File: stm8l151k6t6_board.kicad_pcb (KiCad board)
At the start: 2 copper layers, 68.4 x 39.4 mm, 31 parts, among them J1 Conn_01x08, J2 Conn_01x08, J3 Conn_01x08, J4 Conn_01x08, J5 Conn_01x04, U1 USB_B_Micro, U2 TPMIC5504, U3 STM8L151K6T6, Y1 8MHz, Y2 32K768Hz

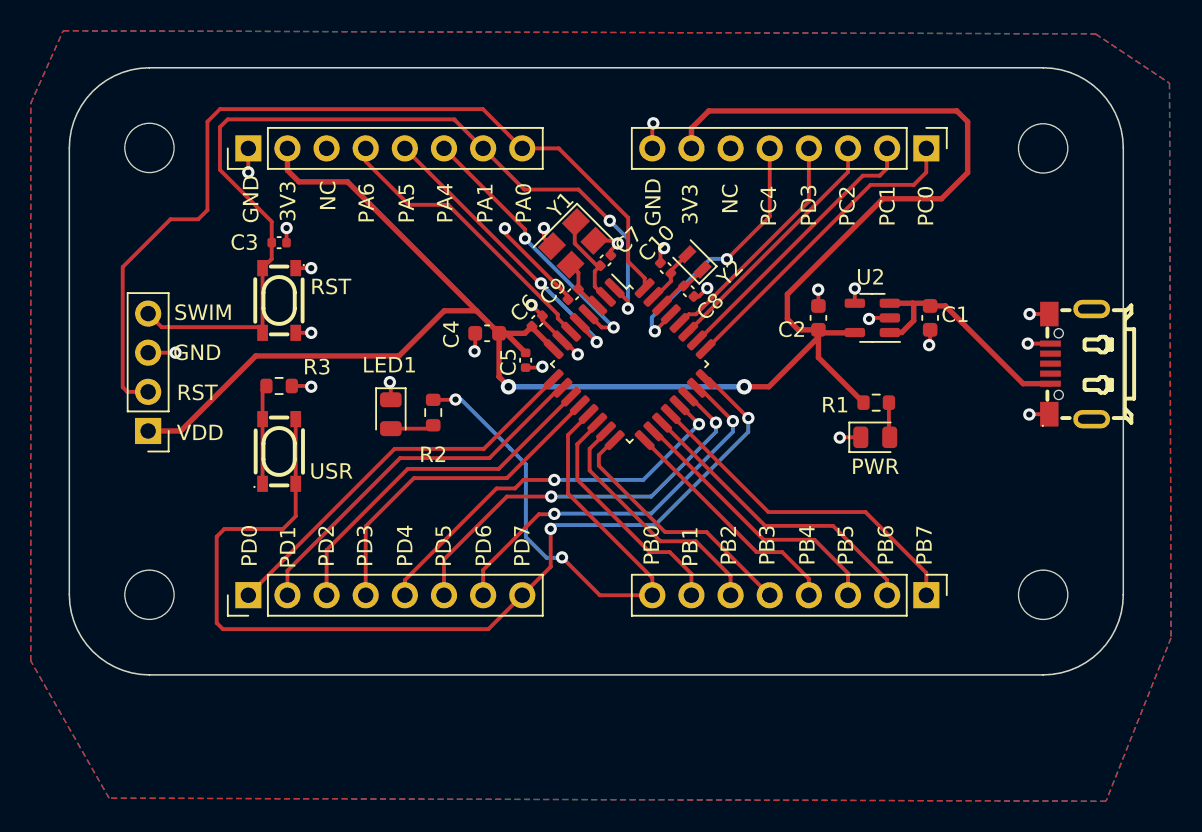
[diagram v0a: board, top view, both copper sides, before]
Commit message: updated version
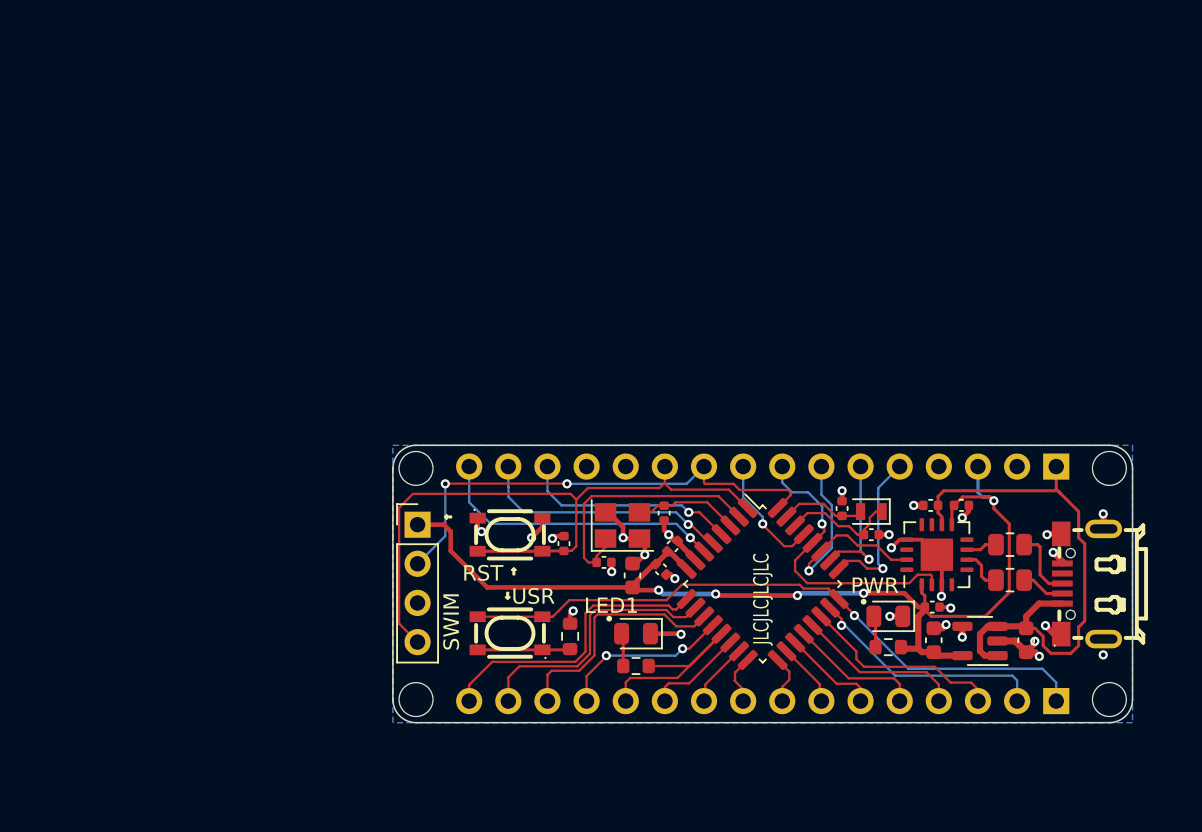
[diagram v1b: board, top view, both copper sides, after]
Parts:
- removed the J2 at (147.6, 113.7)
- removed J4: Conn_01x08, Connector_PinHeader_2.54mm:PinHeader_1x08_P2.54mm_Vertical
- added C1: 100nF, Capacitor_SMD:C_0402_1005Metric, F.Cu at (147.9, 107.9)
- added C3: 100nF, Capacitor_SMD:C_0402_1005Metric, F.Cu at (148.0, 114.5)
- added C6: 100nF, Capacitor_SMD:C_0402_1005Metric, F.Cu at (149.9, 107.9)
- added R2: 27, Resistor_SMD:R_0805_2012Metric, F.Cu at (153.1, 110.5)
- added R3: 27, Resistor_SMD:R_0805_2012Metric, F.Cu at (153.1, 112.8)
- added U3: FT230XQ, Package_DFN_QFN:QFN-16-1EP_4x4mm_P0.65mm_EP2.1x2.1mm, F.Cu at (148.3, 111.1)
- H1, H2, H3, H4: footprint MountingHole:MountingHole_3.2mm_M3 -> MountingHole:MountingHole_2.2mm_M2
- J1, J3: value Conn_01x08 -> Conn_01x16; footprint Connector_PinHeader_2.54mm:PinHeader_1x08_P2.54mm_Vertical -> Connector_PinHeader_2.54mm:PinHeader_1x16_P2.54mm_Vertical; moved to B.Cu
- R1: value 100 -> 1k
- R4: renamed from R2; value 100 -> 1k
- R5: renamed from R3; value 100 -> 1K
- moved H2 71.9 mm to (159.5, 120.5)
- moved J1 56.4 mm to (156.1, 105.4)
- moved H1 54.2 mm to (114.5, 120.5)
- moved J3 36.8 mm to (156.1, 120.6), turned to 90 degrees
- moved C5 26.9 mm to (124.1, 110.4), turned to 90 degrees
- moved R5 24.9 mm to (124.5, 116.4), turned to 90 degrees
- moved C4 22.2 mm to (148.1, 116.7)
- moved U2 22.1 mm to (151.1, 116.7)
- moved C2 21.8 mm to (154.1, 116.7)
- moved D2 21.4 mm to (128.8, 116.2), turned to 180 degrees
- moved SW1 21.3 mm to (120.6, 109.8), turned to 0 degrees
- moved R4 21.1 mm to (128.8, 118.3), turned to 180 degrees
- moved Y2 19.8 mm to (144.1, 108.3), turned to 180 degrees
- moved C12 19.8 mm to (144.1, 109.8), turned to 0 degrees
- moved C10 19.6 mm to (126.7, 111.6), turned to 0 degrees
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- renumbered C7 to C10, C9 to C11, C8 to C12, C10 to C13, C1 to C2, C2 to C4, C3 to C5, C4 to C7, C5 to C8, C6 to C9, PWR to D1, LED1 to D2, J5 to J2, RST to SW1, USR to SW2, U3 to U4
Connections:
- C5 pad 1: /PA1 -> /PA1/RST
- J1 pad 1: GND -> +5V
- J1 pad 2: +3V3 -> GND
- J1 pad 3: unconnected-(J1-Pad3) -> +3V3
- J1 pad 4: /PA6 -> GND
- J1 pad 5: /PA5 -> /PC0
- J1 pad 6: /PA4 -> /PC1
- J1 pad 7: /PA1 -> /USART_RX
- J1 pad 8: /PA0 -> /USART_TX
- J2 pad 2: /PA0 -> /PA0/SWIM
- J2 pad 4: /PA1 -> /PA1/RST
- J3 pad 1: /PC0 -> /PD7
- J3 pad 2: /PC1 -> /PD6
- J3 pad 3: /PC2 -> /PD5
- J3 pad 4: /PC3 -> /PD4
- J3 pad 5: /PC4 -> /PB7
- J3 pad 6: unconnected-(J3-Pad6) -> /PB6
- J3 pad 7: +3V3 -> /PB5
- J3 pad 8: GND -> /PB4
- SW1 pad 3: /PA1 -> /PA1/RST
- SW1 pad 4: /PA1 -> /PA1/RST
- U1 pad 2: unconnected-(U1-Pad2) -> /USB_D+
- U1 pad 3: unconnected-(U1-Pad3) -> /USB_D-
- U4 pad 1: /PA1 -> /PA1/RST
- U4 pad 27: /PC2 -> /USART_RX
- U4 pad 28: /PC3 -> /USART_TX
- U4 pad 32: /PA0 -> /PA0/SWIM
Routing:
- net /PA1: track 58.9 -> 0.00 mm, vias 2 -> 0
- net /PA0: track 57.9 -> 0.00 mm
- net +3V3: track 127.0 -> 69.7 mm, vias 2 -> 5
- net /PA1/RST: track 0.00 -> 44.1 mm
- net /PA0/SWIM: track 0.00 -> 32.2 mm, vias 0 -> 2
- net /PB0: track 37.1 -> 14.3 mm, vias 2 -> 0
- net /PD7: track 63.8 -> 42.3 mm, vias 2 -> 1
- net +5V: track 15.6 -> 36.7 mm
- net /USART_TX: track 0.00 -> 19.4 mm, vias 0 -> 1
- net /PC2: track 16.4 -> 0.00 mm
- net /USART_RX: track 0.00 -> 15.9 mm, vias 0 -> 1
- net /PD4: track 26.0 -> 10.9 mm, vias 2 -> 0
- net /PC3: track 15.1 -> 0.00 mm
- net /PB5: track 17.9 -> 4.19 mm
- net /PB7: track 22.3 -> 8.68 mm
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- removed copper zone on F.Cu, net GND
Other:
- board size 68.4 x 39.4 mm -> 48 x 18 mm
- board text added: "5V"
- board text added: "Andres Bravo v2.0"
- board text added: "JLCJLCJLCJLC"
- board text added: "LED1"
- board text added: "PWR"
- board text added: "RX"
- board text added: "STM8L151K6T6 DEVELOPMENT BOARD"
- board text added: "TX"
- board text added: "USR"
- board text removed: "PC2"
- board text removed: "STM8L151K6T6 DEVELOPMENT BOARD ANDRES BRAVO V1.0"
- board text removed: "VDD"
